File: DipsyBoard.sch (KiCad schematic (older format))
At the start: 39 parts, among them CON1 SDMMC_Card, P1 USB_OTG, P2 Analog, P3 Digital, P4 JLINK-SWD, P5 POWER, P6 CORTEX-JTAG, SW1 SW_PUSH, U1 STM32L486Rx-LQFP64, U2 NCP1117ST33T3G, U3 APX823, U4 PUSBM5V5X4, X1 XTAL, Y1 Crystal

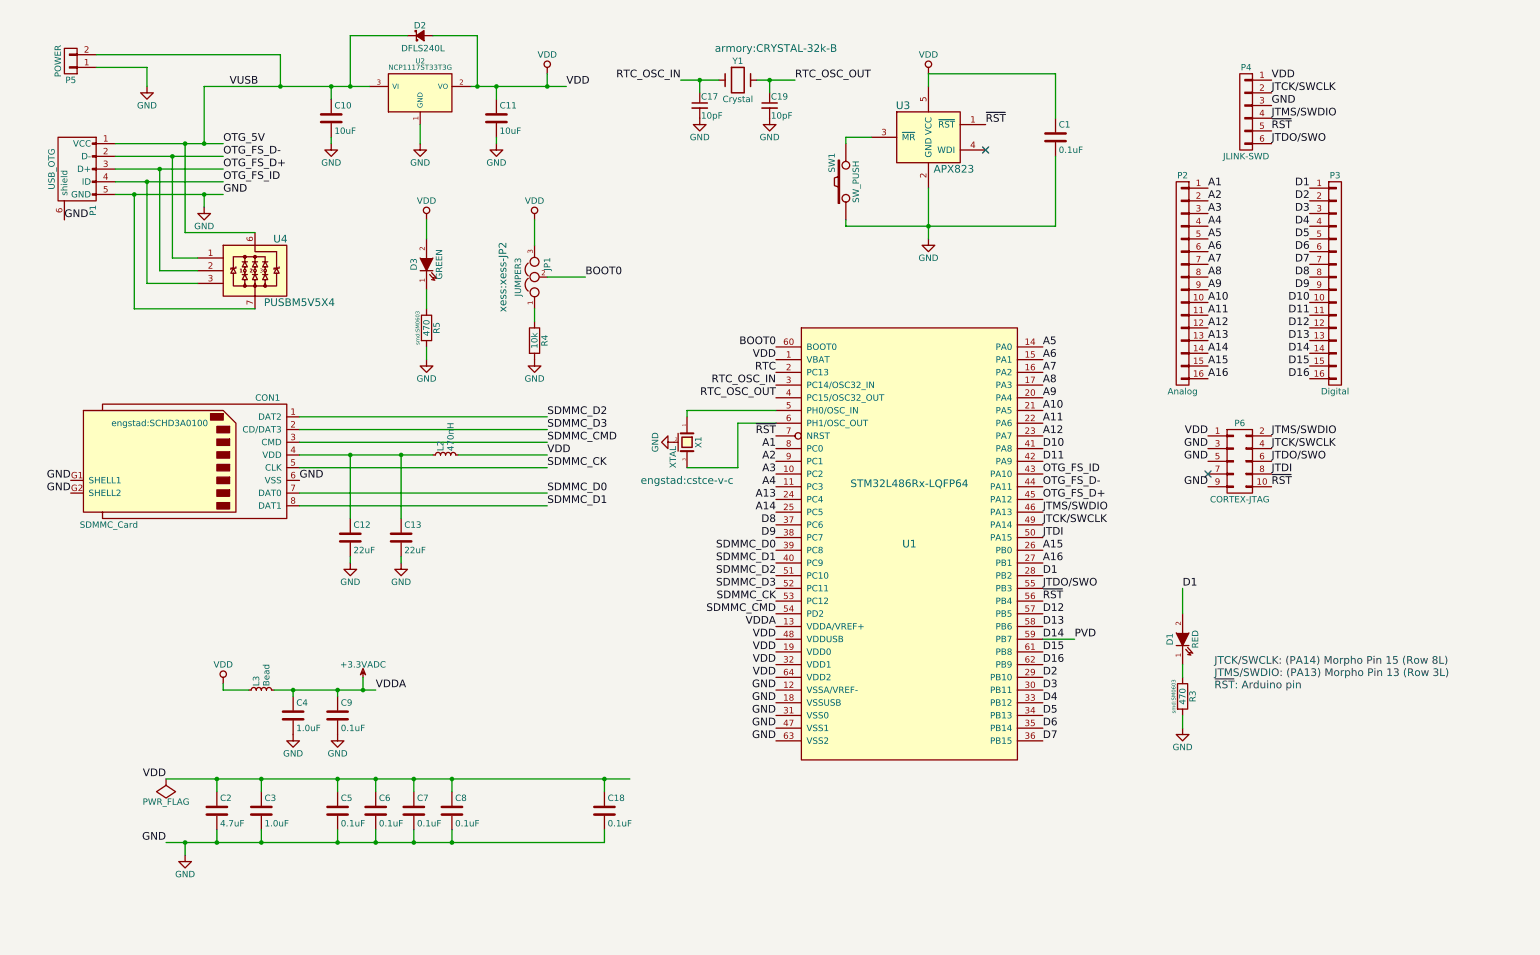
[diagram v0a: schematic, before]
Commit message: More work
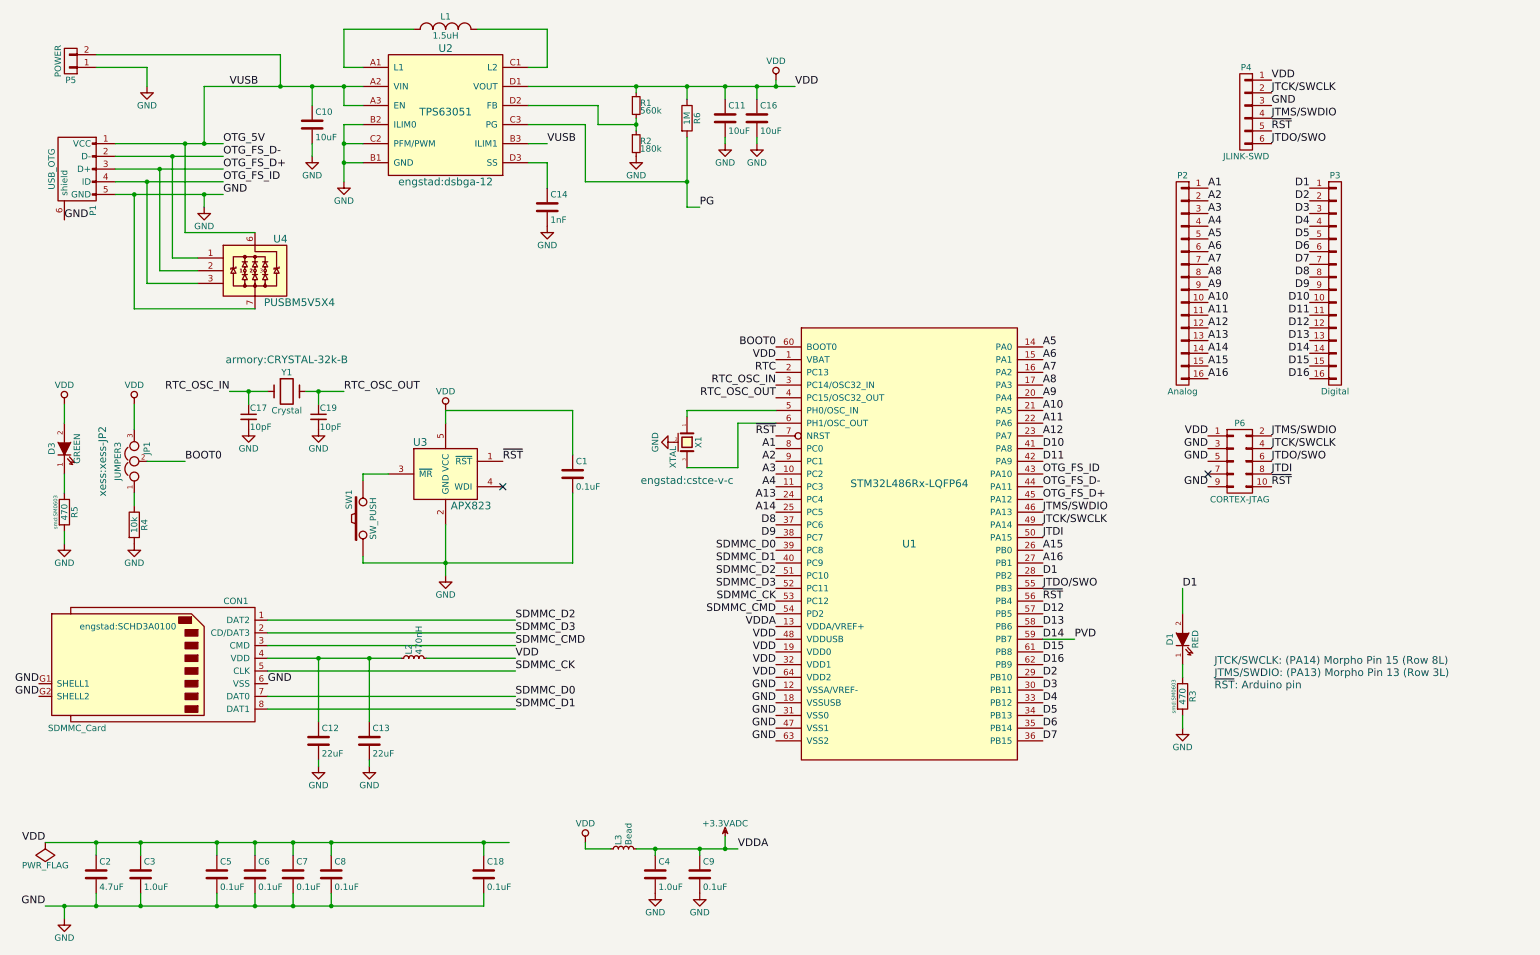
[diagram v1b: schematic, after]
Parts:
- removed D2: DFLS240L, engstad:diode-smd-powerdi-123, symbol D_Schottky_Small
- removed U2: NCP1117ST33T3G, TO_SOT_Packages_SMD:SOT-223, symbol NCP1117ST33T3G
- added C14: 1nF, smd:SM0603, symbol C
- added C16: 10uF, smd:SM0805, symbol C
- added L1: 1.5uH, engstad:inductor-smd-1212, symbol INDUCTOR_SMALL
- added R1: 560k, smd:SM0603, symbol R_Small
- added R2: 180k, smd:SM0603, symbol R_Small
- added R6: 1M, smd:SM0603, symbol R
- added U2: TPS63051, engstad:dsbga-12, symbol TPS63051
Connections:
- net GND: now also C14.2, C16.2, R2.2, U2.B1 (GND), U2.B2 (ILIM0), U2.C2 (PFM/PWM)
- net OTG_5V: now also U2.A2 (VIN), U2.A3 (EN), U2.B3 (ILIM1)
- net VDD: now also C16.1, R1.1, R6.1, U2.D1 (VOUT)
- new net: L1.1, U2.A1 (L1)
- new net: L1.2, U2.C1 (L2)
- new net: R1.2, R2.1, U2.D2 (FB)
- new net: C14.1, U2.D3 (SS)
- new net PG: R6.2, U2.C3 (PG)
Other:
- moved on the sheet: C1, C10, C11, C12, C13, C17, C18, C19, C2, C3, C4, C5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
